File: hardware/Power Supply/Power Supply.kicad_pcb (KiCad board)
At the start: 2 copper layers, 100 x 71 mm, 21 parts, among them J1 230 Vac, J2 12V, J3 8V, U4 L7808CV

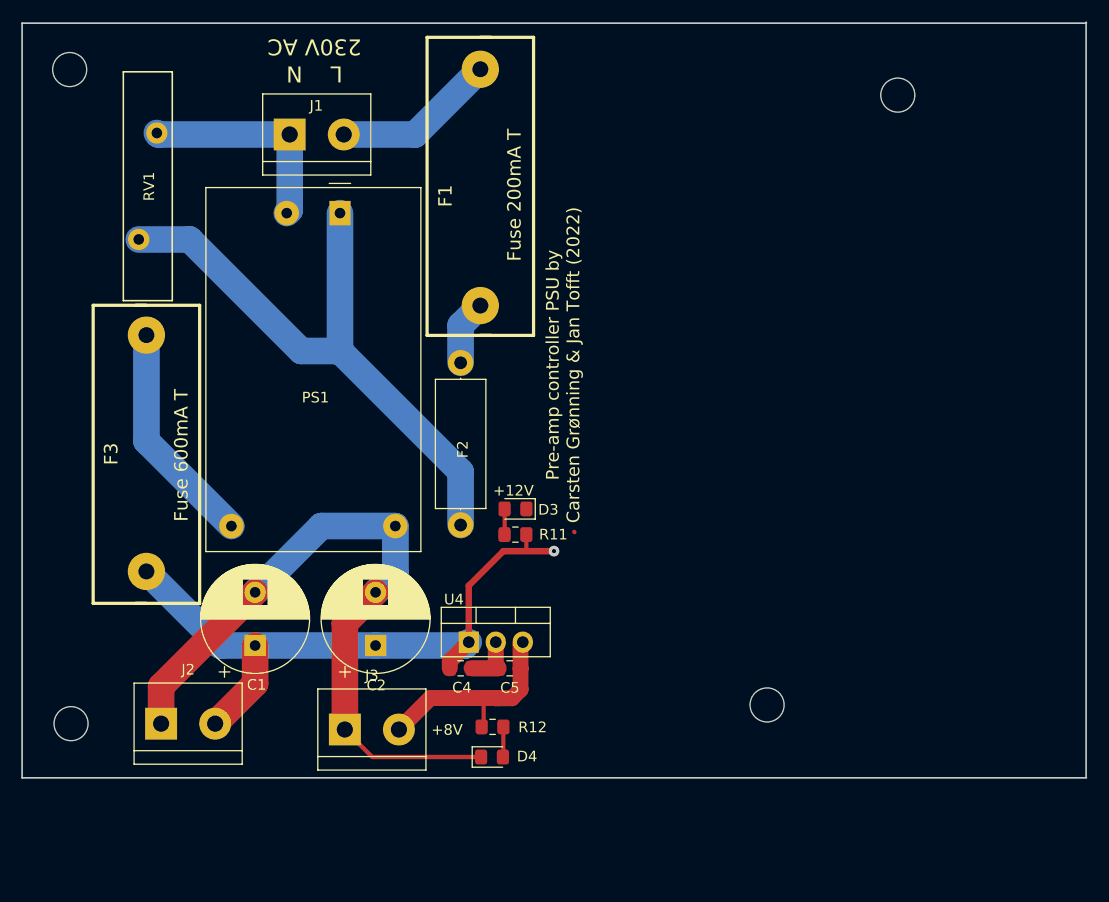
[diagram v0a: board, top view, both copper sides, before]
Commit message: psu pcb ready
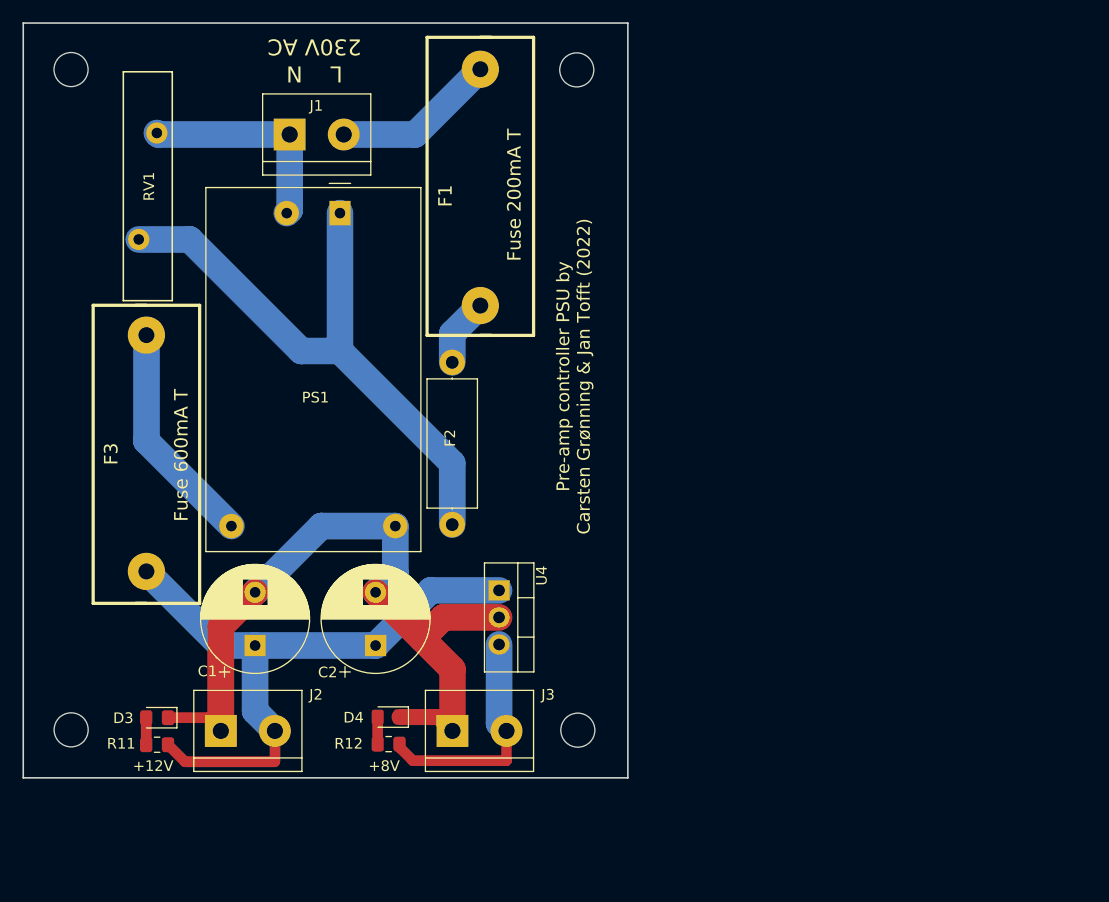
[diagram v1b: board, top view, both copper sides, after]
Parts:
- removed C4: 0.33uF, Capacitor_SMD:C_0805_2012Metric_Pad1.15x1.40mm_HandSolder
- removed C5: 0.1uF, Capacitor_SMD:C_0805_2012Metric_Pad1.15x1.40mm_HandSolder
- moved R11 39.0 mm to (105.8, 137.3)
- moved D3 39.0 mm to (105.8, 134.8)
- moved REF** 30.3 mm to (145.2, 73.9)
- moved REF** 17.9 mm to (145.3, 135.9)
- moved F2 15.3 mm to (133.5, 101.4), turned to -90 degrees
- moved D4 10.4 mm to (127.5, 134.7), turned to 180 degrees
- moved J3 10.1 mm to (133.5, 136.0)
- moved R12 9.90 mm to (127.5, 137.2), turned to 0 degrees
- moved J2 5.65 mm to (111.8, 136.0)
- moved U4 5.63 mm to (137.9, 122.8), turned to -90 degrees
- moved REF** 0.58 mm to (97.7, 135.9)
- moved REF** 0.13 mm to (97.7, 73.9)
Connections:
- F2 pad 2: Net-(F1-Pad2) -> Net-(F2-Pad2)
- PS1 pad 1: Net-(F1-Pad2) -> Net-(F2-Pad2)
- RV1 pad 1: Net-(F1-Pad2) -> Net-(F2-Pad2)
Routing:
- net Net-(F1-Pad2): track 64.6 -> 6.43 mm
- net Net-(F2-Pad2): track 0.00 -> 56.9 mm
- net +12V: track 62.1 -> 60.5 mm, vias 1 -> 0
- net +8V: track 20.9 -> 22.1 mm
- net GND: track 71.5 -> 72.2 mm
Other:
- board size 100 x 71 mm -> 56.8 x 70.9 mm

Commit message: mod psu + control v 0.25
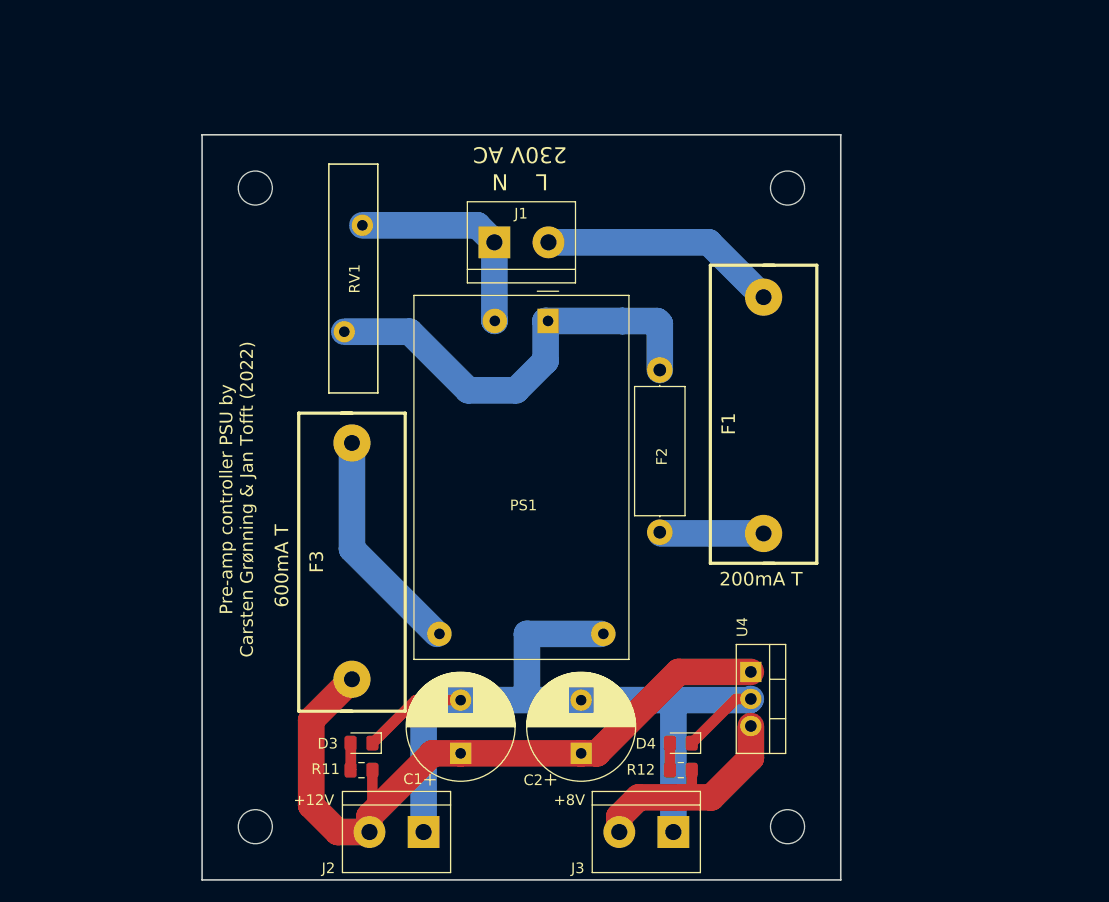
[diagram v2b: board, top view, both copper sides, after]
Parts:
- F1: value Fuse 200mA T -> 200mA T
- F3: value Fuse 600mA T -> 600mA T
- moved F1 34.2 mm to (162.8, 106.2)
- moved D4 27.6 mm to (155.0, 137.2)
- moved R12 27.6 mm to (155.0, 139.7)
- moved F2 25.2 mm to (153.0, 117.3), turned to 90 degrees
- moved U4 24.9 mm to (161.6, 130.5)
- moved J3 22.8 mm to (154.3, 145.5), turned to 180 degrees
- moved REF** 22.7 mm to (165.0, 85.0)
- moved PS1 22.0 mm to (142.5, 97.5)
- moved C2 21.8 mm to (145.6, 138.1)
- moved F3 21.8 mm to (124.1, 120.2)
- moved C1 21.8 mm to (134.3, 138.1)
- moved J1 21.7 mm to (137.5, 90.1)
- moved REF** 21.7 mm to (165.0, 145.0)
- moved J2 21.3 mm to (130.8, 145.5), turned to 180 degrees
- moved RV1 21.2 mm to (123.4, 98.5)
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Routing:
- net Net-(F2-Pad2): track 56.9 -> 41.3 mm
- net GND: track 72.2 -> 85.5 mm
- net +12V: track 60.5 -> 68.8 mm
- net Net-(F1-Pad1): track 15.4 -> 22.3 mm
- net Net-(F1-Pad2): track 6.43 -> 9.63 mm
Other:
- board size 56.8 x 70.9 mm -> 60 x 70 mm
